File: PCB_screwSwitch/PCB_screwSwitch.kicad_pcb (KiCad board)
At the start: 4 copper layers, 39 x 15 mm, 3 parts, among them J1 XT30PW-M, J2 Screw_Terminal_01x02

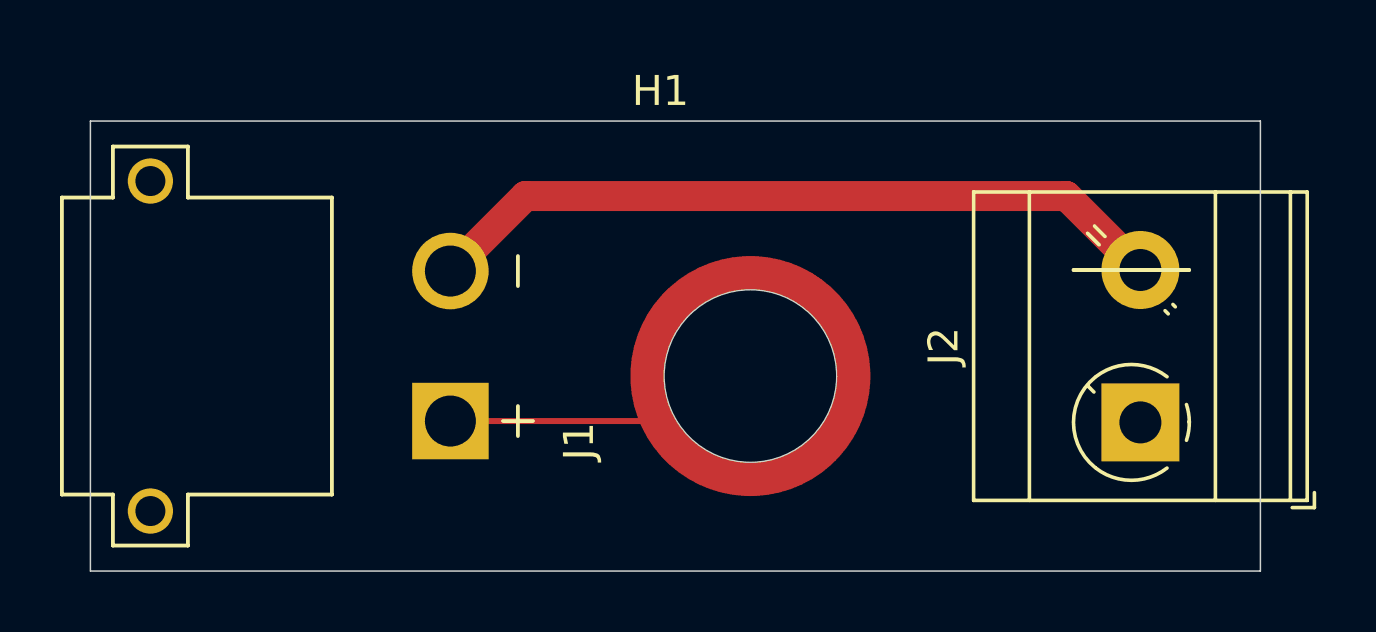
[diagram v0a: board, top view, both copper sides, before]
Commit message: Rev 3
Created rev A of custom PCB Switch
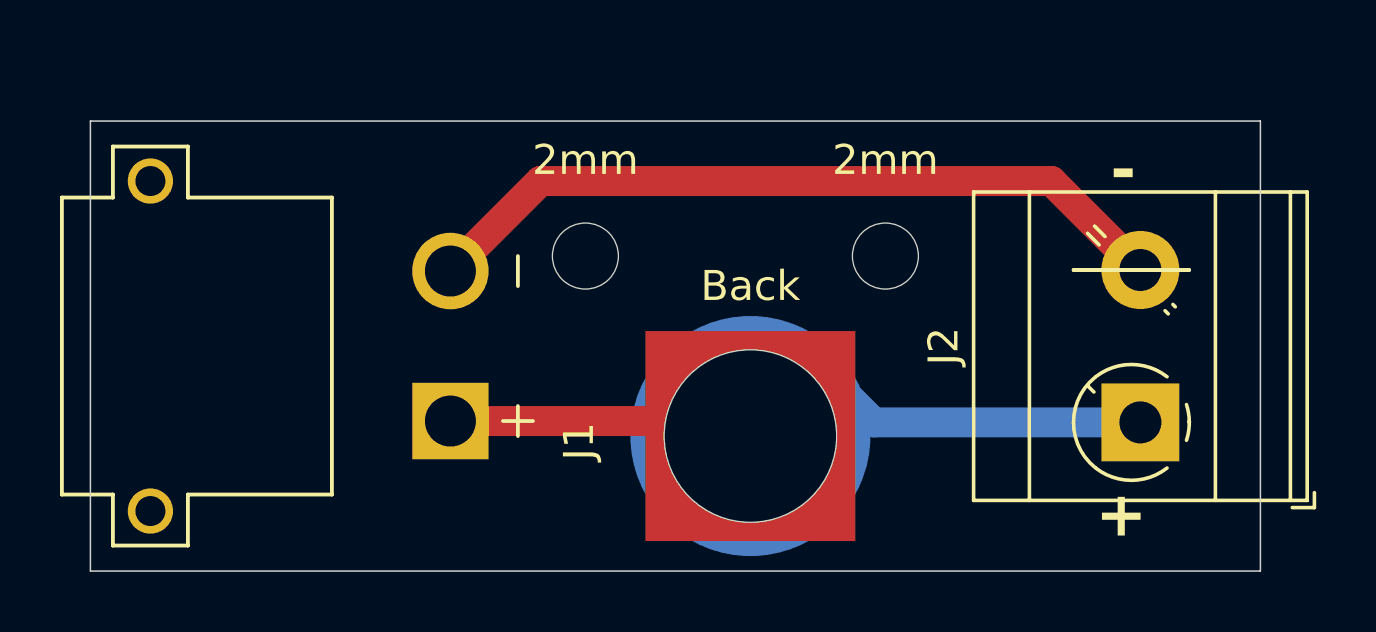
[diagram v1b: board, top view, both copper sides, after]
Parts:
- added 2mm: MountingHole_2.2mm_M2, MountingHole:MountingHole_2.2mm_M2, F.Cu at (167.0, 79.0)
- added 2mm: MountingHole_2.2mm_M2, MountingHole:MountingHole_2.2mm_M2, F.Cu at (157.0, 79.0)
- added Front: hole_center, parts_footprints:hole_center, F.Cu at (162.5, 85.0)
- added H2: MountingHole_Pad, parts_footprints:hole_bottom, F.Cu at (162.5, 85.0)
- moved Back 2.00 mm to (162.5, 85.0)
- renumbered H1 to Back
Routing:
- net Net-(J2-Pin_1): track 0.00 -> 11.5 mm
- net Net-(H1-Pad1): track 8.04 -> 11.7 mm
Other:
- copper layers 4 -> 2
- board text added: "+"
- board text added: "-"
- board text added: "Batt"
- board text added: "Rev A"
- board text added: "XT-30 Screwswitch"
